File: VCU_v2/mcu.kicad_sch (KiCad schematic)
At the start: 33 parts, among them SW1 SW_Push, U5 STM32H723ZGT6, Y1 16 MHz, Y2 32.768 kHz

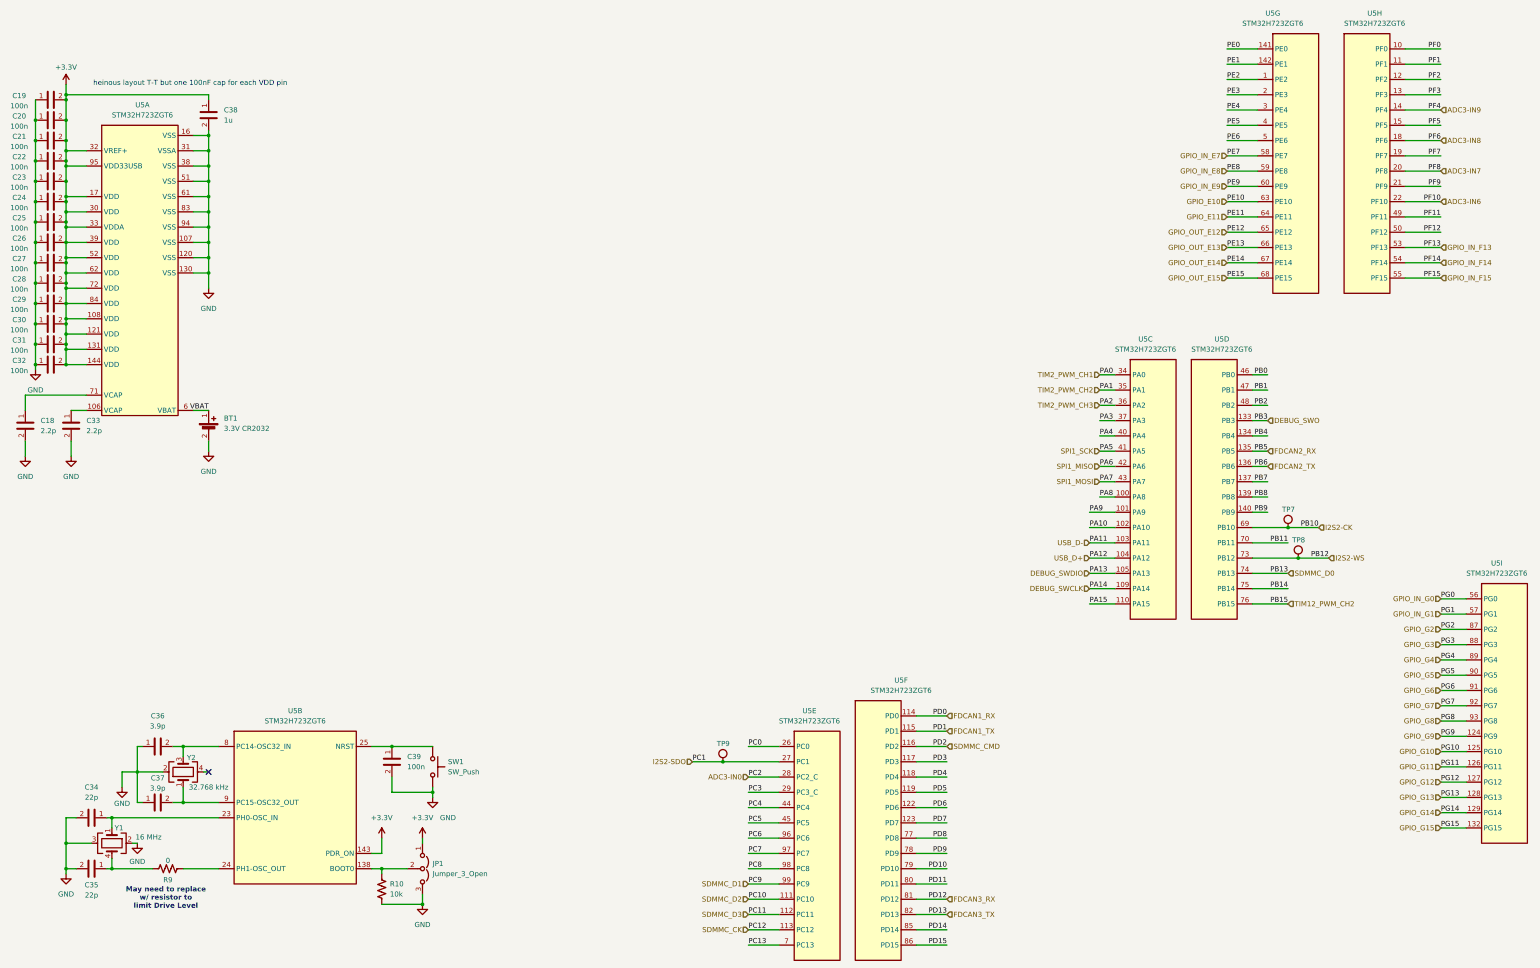
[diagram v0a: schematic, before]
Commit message: vcu v2 schematics done
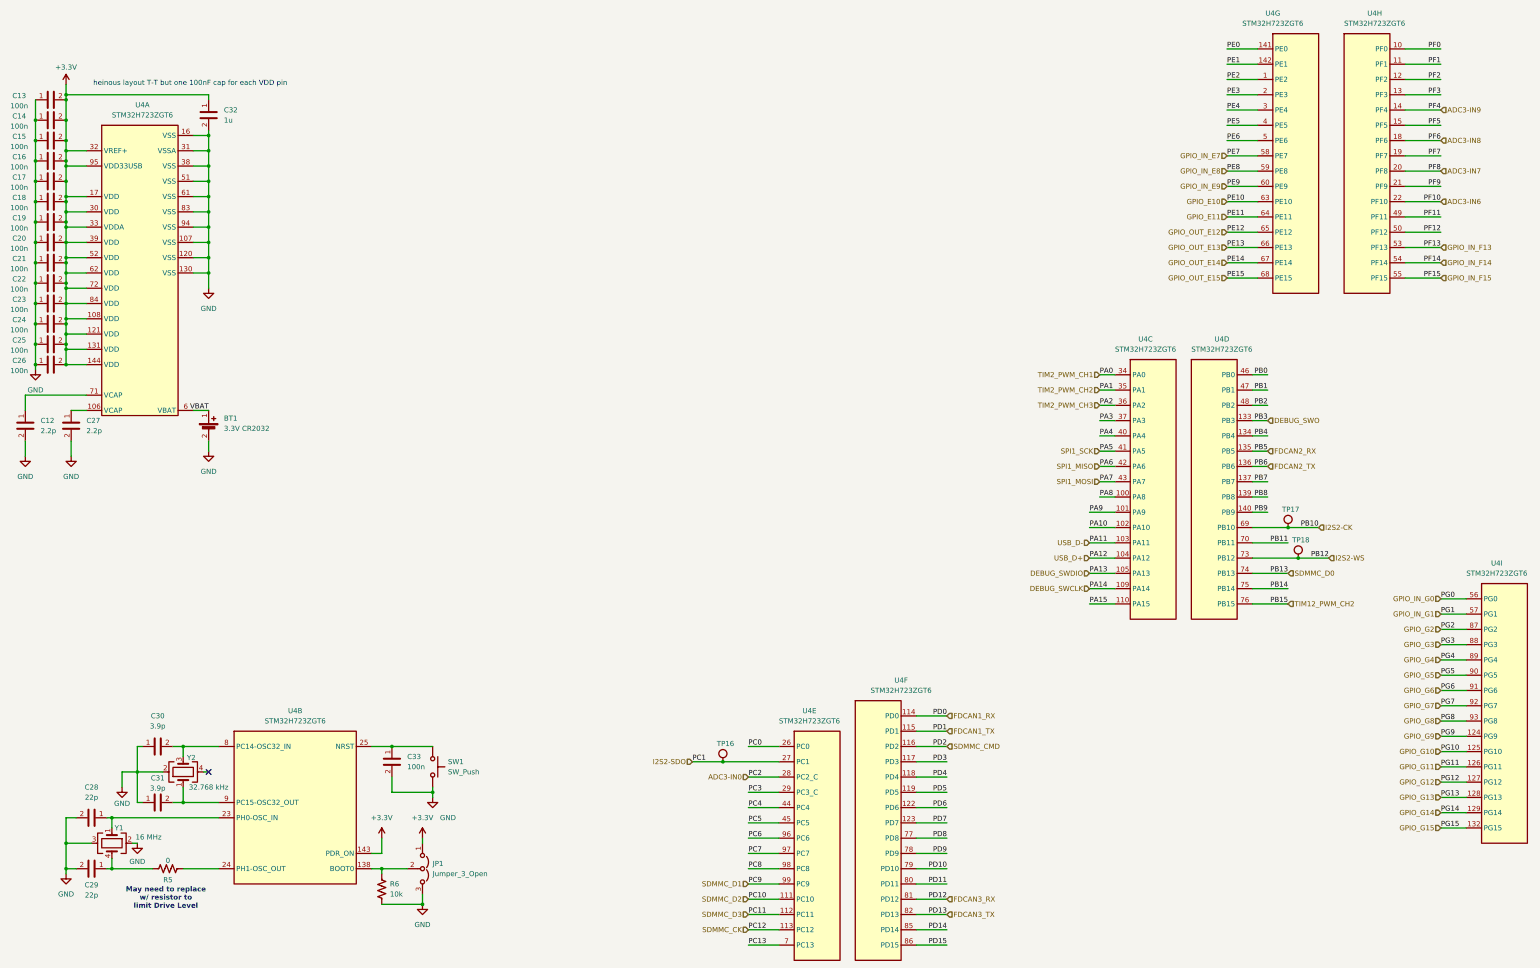
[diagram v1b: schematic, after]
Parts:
- renumbered C18 to C12, C19 to C13, C20 to C14, C21 to C15, C22 to C16, C23 to C17, C24 to C18, C25 to C19, C26 to C20, C27 to C21, C28 to C22, C29 to C23, C30 to C24, C31 to C25, C32 to C26, C33 to C27, C34 to C28, C35 to C29, C36 to C30, C37 to C31, C38 to C32, C39 to C33, R9 to R5, R10 to R6, TP9 to TP16, TP7 to TP17, TP8 to TP18, U5 to U4

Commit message: placements friggin 80% friggin done shoutout epstein
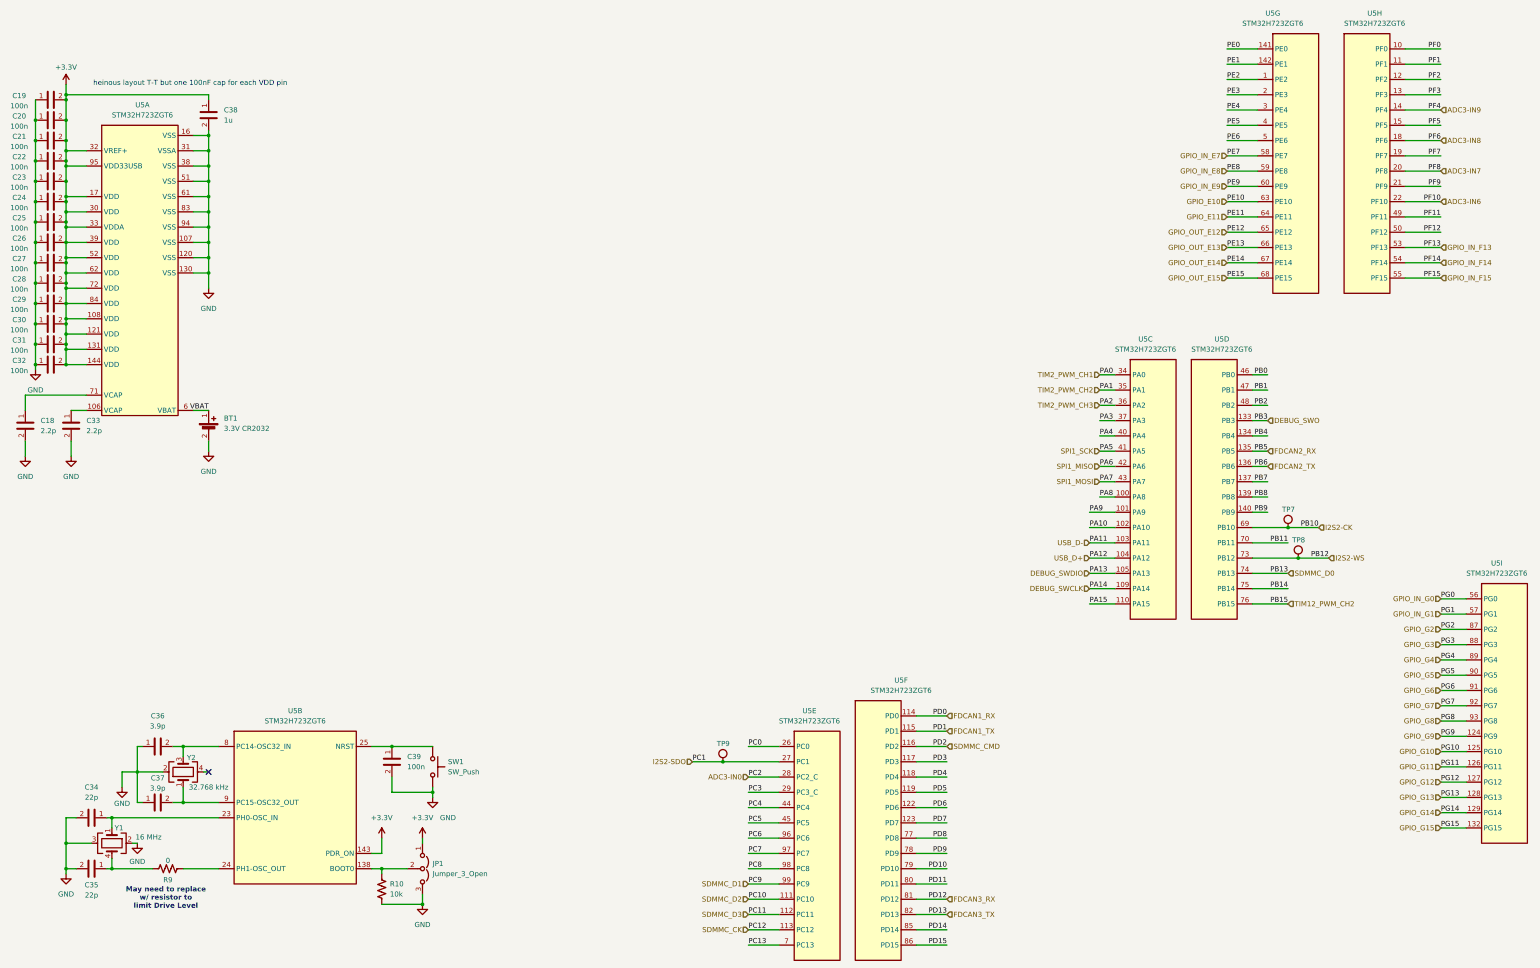
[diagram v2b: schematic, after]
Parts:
- renumbered C12 to C18, C13 to C19, C14 to C20, C15 to C21, C16 to C22, C17 to C23, C18 to C24, C19 to C25, C20 to C26, C21 to C27, C22 to C28, C23 to C29, C24 to C30, C25 to C31, C26 to C32, C27 to C33, C28 to C34, C29 to C35, C30 to C36, C31 to C37, C32 to C38, C33 to C39, R6 to R10, R5 to R9, TP17 to TP7, TP18 to TP8, TP16 to TP9, U4 to U5
